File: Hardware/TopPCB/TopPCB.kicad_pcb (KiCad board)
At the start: 4 copper layers, 9.6 x 11.6 mm, 9 parts

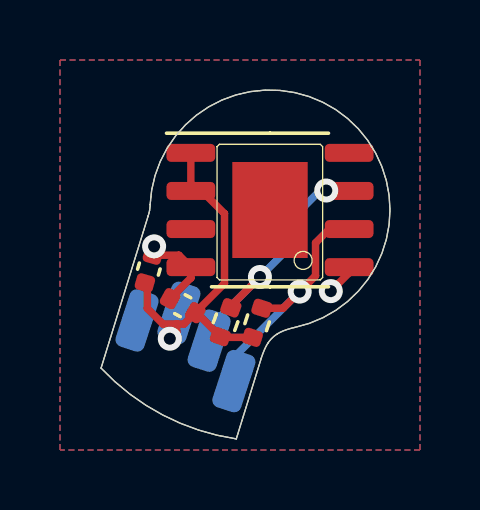
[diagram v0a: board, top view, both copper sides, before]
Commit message: updated gerbers
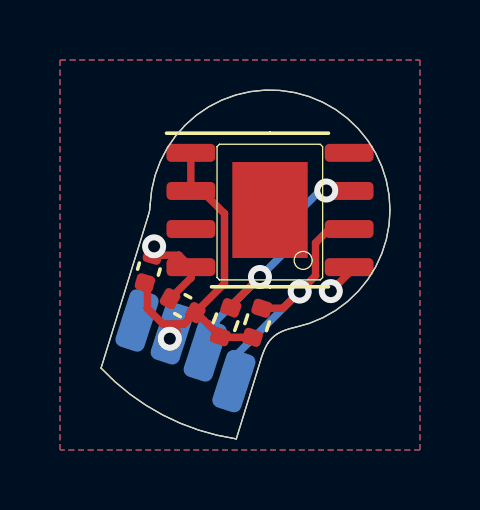
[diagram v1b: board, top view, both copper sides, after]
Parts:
- moved ? 0.72 mm to (76.7, 44.1)
- moved ? 0.35 mm to (77.8, 44.7)
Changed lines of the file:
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@@
   )
   (footprint "" (layer "F.Cu")
-    (at 77.970164 44.355542)
+    (at 77.84 44.68)
     (fp_text reference "" (at 0 0) (layer "F.SilkS")
         (effects (font (size 1.27 1.27) (thickness 0.15)))
@@
   )
   (footprint "" (layer "F.Cu")
-    (at 76.964196 43.427148)
+    (at 76.74 44.11)
     (fp_text reference "" (at 0 0) (layer "F.SilkS")
         (effects (font (size 1.27 1.27) (thickness 0.15)))
@@
   (via (at 79.664848 42.23272) (size 0.8) (drill 0.4) (layers "F.Cu" "B.Cu") (net 3))
   (via (at 81.875695 39.350563) (size 0.8) (drill 0.4) (layers "F.Cu" "B.Cu") (net 3))
-  (segment (start 77.970164 44.355542) (end 77.970164 43.927404) (width 0.25) (layer "B.Cu") (net 3))
+  (segment (start 77.970164 44.355542) (end 78.19 44.135706) (width 0.25) (layer "B.Cu") (net 3))
   (segment (start 81.67131 39.350563) (end 81.875695 39.350563) (width 0.25) (layer "B.Cu") (net 3))
-  (segment (start 77.970164 43.927404) (end 79.664848 42.23272) (width 0.25) (layer "B.Cu") (net 3))
+  (segment (start 78.19 43.707568) (end 79.664848 42.23272) (width 0.25) (layer "B.Cu") (net 3))
   (segment (start 79.664848 42.23272) (end 81 40.897568) (width 0.25) (layer "B.Cu") (net 3))
+  (segment (start 78.19 44.135706) (end 78.19 43.707568) (width 0.25) (layer "B.Cu") (net 3))
   (segment (start 81 40.021873) (end 81.67131 39.350563) (width 0.25) (layer "B.Cu") (net 3))
   (segment (start 81 40.897568) (end 81 40.021873) (width 0.25) (layer "B.Cu") (net 3))

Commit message: updated ibom
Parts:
- U1: value ~ -> AS5600
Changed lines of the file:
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@@
         (effects (font (size 1 1) (thickness 0.15)))
     )
-    (fp_text value "~" (at 0 3.4) (layer "F.Fab")
+    (fp_text value "AS5600" (at 0 3.4) (layer "F.Fab")
         (effects (font (size 1 1) (thickness 0.15)))
     )
@@
   (footprint "" (layer "B.Cu")
     (at 75.567872 43.681249 162)
+    (attr exclude_from_bom)
     (fp_text reference "" (at 0 0 162) (layer "B.SilkS")
         (effects (font (size 1.27 1.27) (thickness 0.15)) (justify mirror))
